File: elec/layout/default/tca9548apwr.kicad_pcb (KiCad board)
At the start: 2 copper layers, 225.7 x 100.8 mm, 0 parts

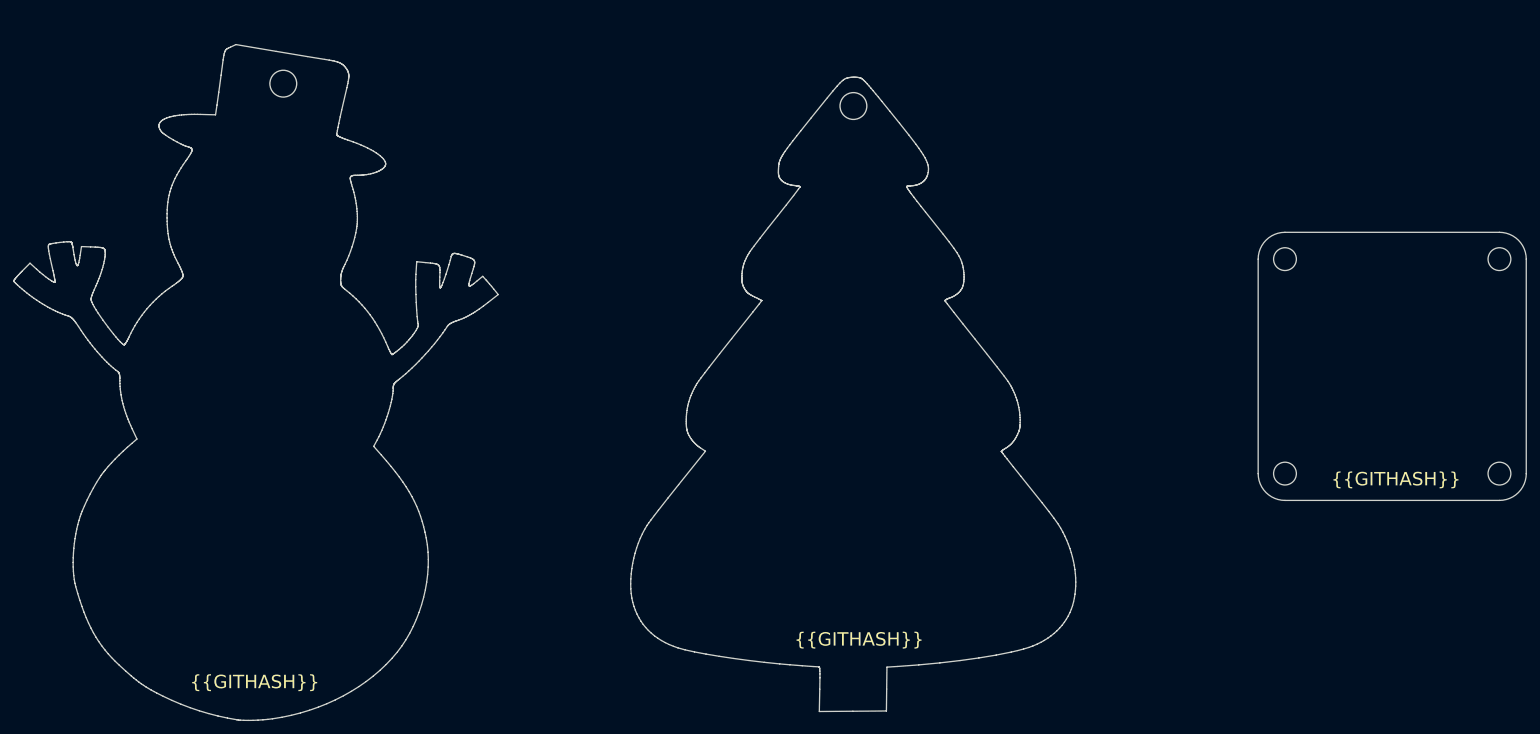
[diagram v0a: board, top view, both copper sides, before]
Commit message: layout
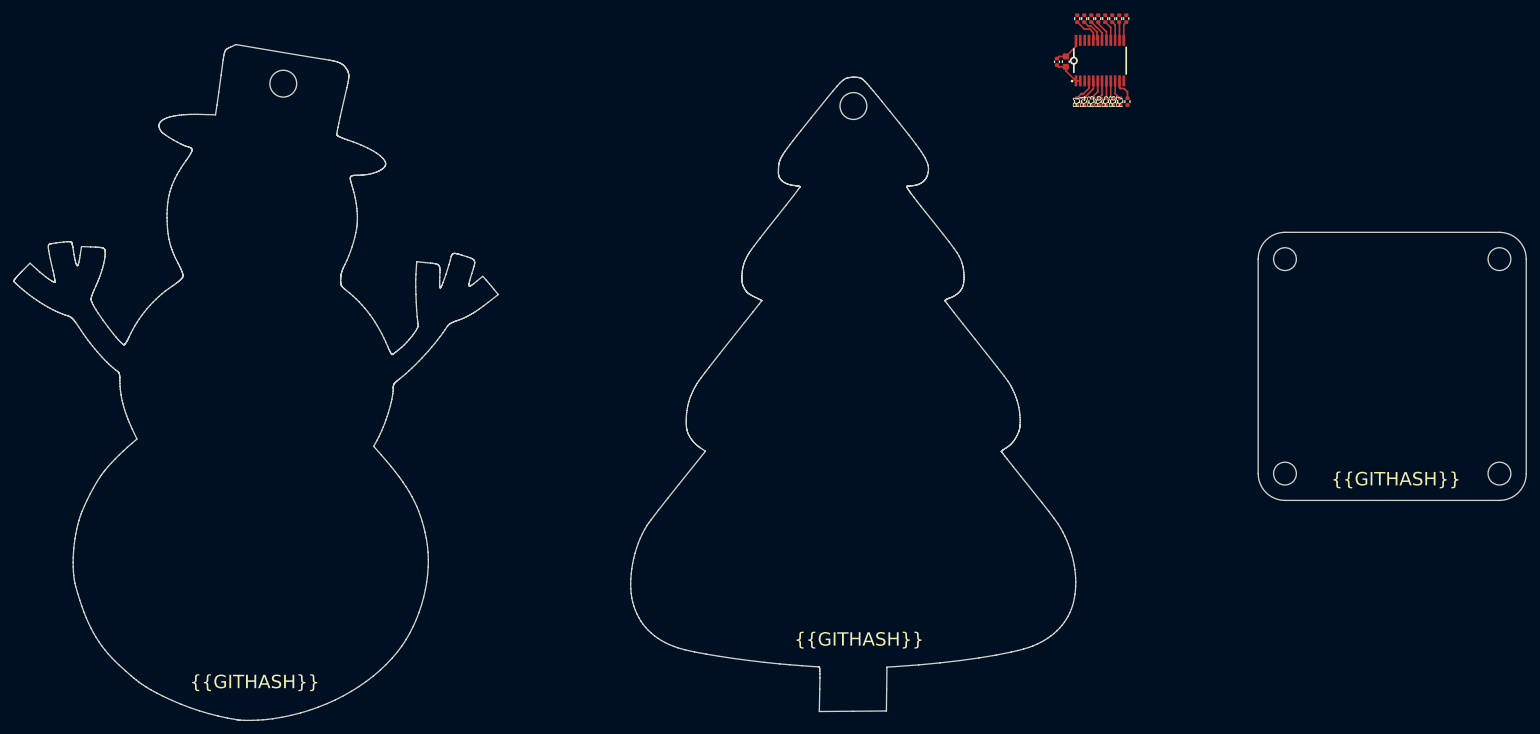
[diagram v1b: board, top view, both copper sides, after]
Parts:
- added C1: Multilayer Ceramic Capacitors MLCC - SMD/SMT 100nF 10V 0402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, lib:C0402, F.Cu at (191.6, 52.3)
- added C2: Multilayer Ceramic Capacitors MLCC - SMD/SMT 2.2uF 10V 0603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, lib:C0603, F.Cu at (192.9, 52.3)
- added R1: Chip Resistor - Surface Mount 10KOhms ±5% 1/16W 0402 RoHS, lib:R0402, F.Cu at (195.7, 58.3)
- added R10: Chip Resistor - Surface Mount 10KOhms ±5% 1/16W 0402 RoHS, lib:R0402, F.Cu at (201.9, 45.9)
- added R11: Chip Resistor - Surface Mount 10KOhms ±5% 1/16W 0402 RoHS, lib:R0402, F.Cu at (198.8, 45.9)
- added R12: Chip Resistor - Surface Mount 10KOhms ±5% 1/16W 0402 RoHS, lib:R0402, F.Cu at (199.9, 45.9)
- added R13: Chip Resistor - Surface Mount 10KOhms ±5% 1/16W 0402 RoHS, lib:R0402, F.Cu at (196.7, 45.9)
- added R14: Chip Resistor - Surface Mount 10KOhms ±5% 1/16W 0402 RoHS, lib:R0402, F.Cu at (197.8, 45.9)
- added R15: Chip Resistor - Surface Mount 10KOhms ±5% 1/16W 0402 RoHS, lib:R0402, F.Cu at (194.6, 45.9)
- added R16: Chip Resistor - Surface Mount 10KOhms ±5% 1/16W 0402 RoHS, lib:R0402, F.Cu at (195.7, 45.9)
- added R2: Chip Resistor - Surface Mount 10KOhms ±5% 1/16W 0402 RoHS, lib:R0402, F.Cu at (194.6, 58.3)
- added R3: Chip Resistor - Surface Mount 10KOhms ±5% 1/16W 0402 RoHS, lib:R0402, F.Cu at (197.8, 58.3)
- added R4: Chip Resistor - Surface Mount 10KOhms ±5% 1/16W 0402 RoHS, lib:R0402, F.Cu at (196.7, 58.3)
- added R5: Chip Resistor - Surface Mount 10KOhms ±5% 1/16W 0402 RoHS, lib:R0402, F.Cu at (200.0, 58.3)
- added R6: Chip Resistor - Surface Mount 10KOhms ±5% 1/16W 0402 RoHS, lib:R0402, F.Cu at (198.9, 58.3)
- added R7: Chip Resistor - Surface Mount 10KOhms ±5% 1/16W 0402 RoHS, lib:R0402, F.Cu at (202.1, 58.3)
- added R8: Chip Resistor - Surface Mount 10KOhms ±5% 1/16W 0402 RoHS, lib:R0402, F.Cu at (201.0, 58.3)
- added R9: Chip Resistor - Surface Mount 10KOhms ±5% 1/16W 0402 RoHS, lib:R0402, F.Cu at (200.9, 45.9)
- added U1: , lib:TSSOP-24_L7.8-W4.4-P0.65-LS6.4-BL, F.Cu at (198.0, 52.2)
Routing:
- net gnd: track 0.00 -> 4.80 mm
- net vcc: track 0.00 -> 4.48 mm
- net scl-7: track 0.00 -> 4.21 mm
- net sda-7: track 0.00 -> 3.89 mm
- net sda: track 0.00 -> 3.51 mm
- net scl-3: track 0.00 -> 3.42 mm
- net scl-6: track 0.00 -> 3.40 mm
- net sda-6: track 0.00 -> 3.24 mm
- net scl: track 0.00 -> 3.13 mm
- net scl-5: track 0.00 -> 3.07 mm
- net sda-1: track 0.00 -> 2.99 mm
- net sda-3: track 0.00 -> 2.94 mm
- net sda-5: track 0.00 -> 2.91 mm
- net sda-4: track 0.00 -> 2.89 mm
- net scl-1: track 0.00 -> 2.84 mm
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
